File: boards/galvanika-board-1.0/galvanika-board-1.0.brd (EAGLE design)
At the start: 100 x 100 mm, 96 parts, among them IC1 LM358D, IC2 7805DT, IC3 74HCT595D, IC4 74HCT595D, IC5 74HCT595D, IC6 ATMEGA48/88/168-PU, IC7 74HC595D, Q1 20MHz

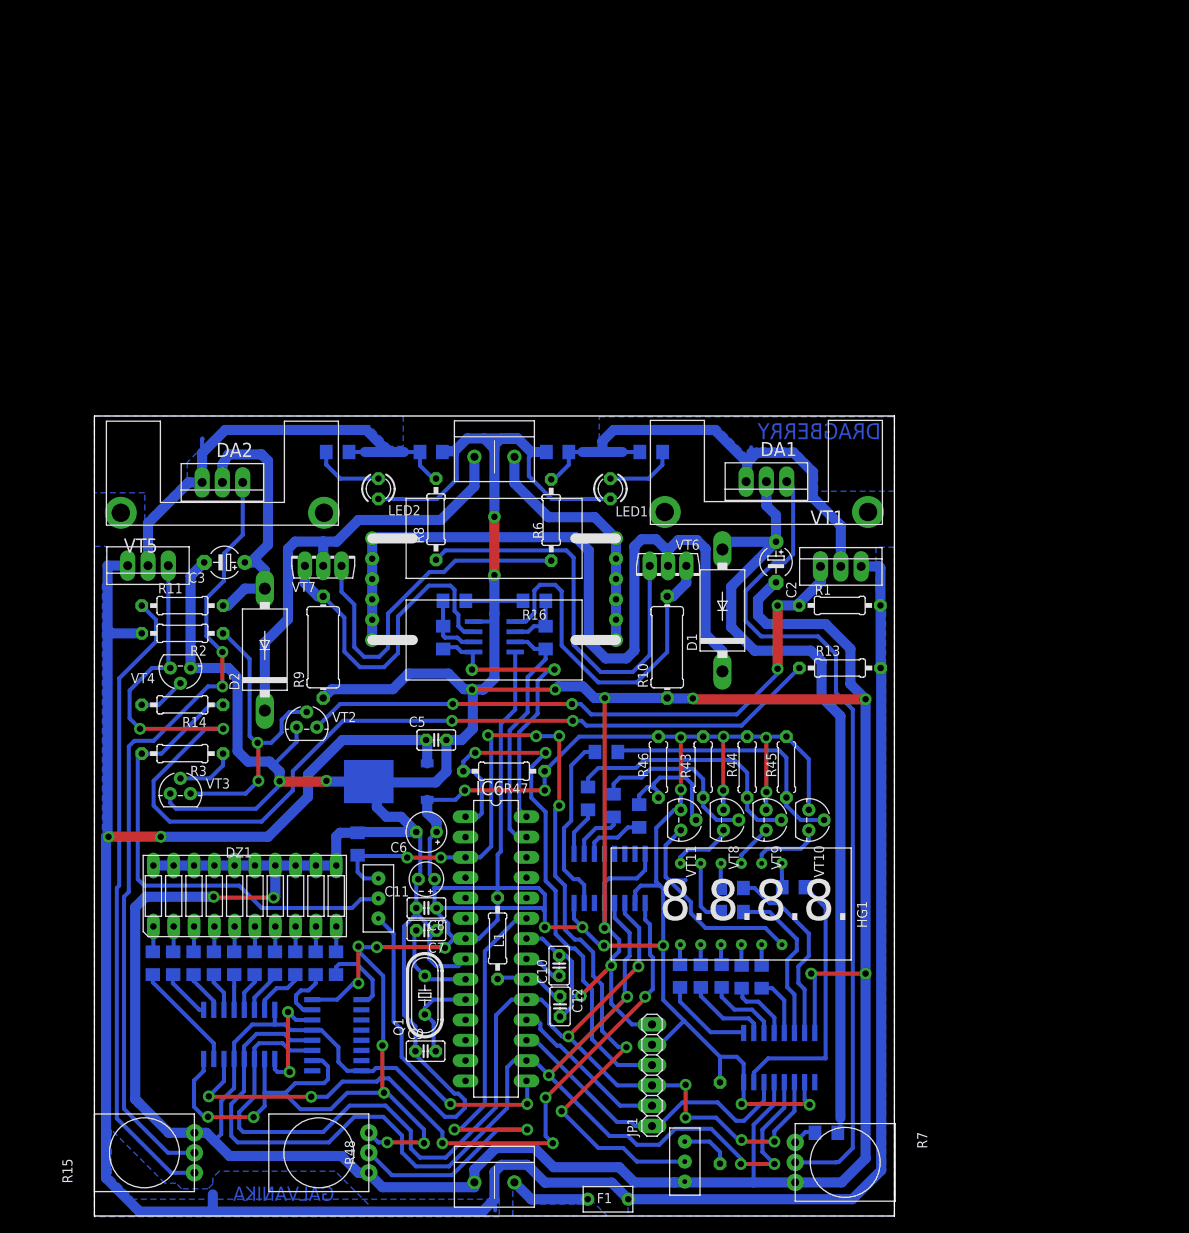
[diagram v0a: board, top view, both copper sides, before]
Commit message: new board version
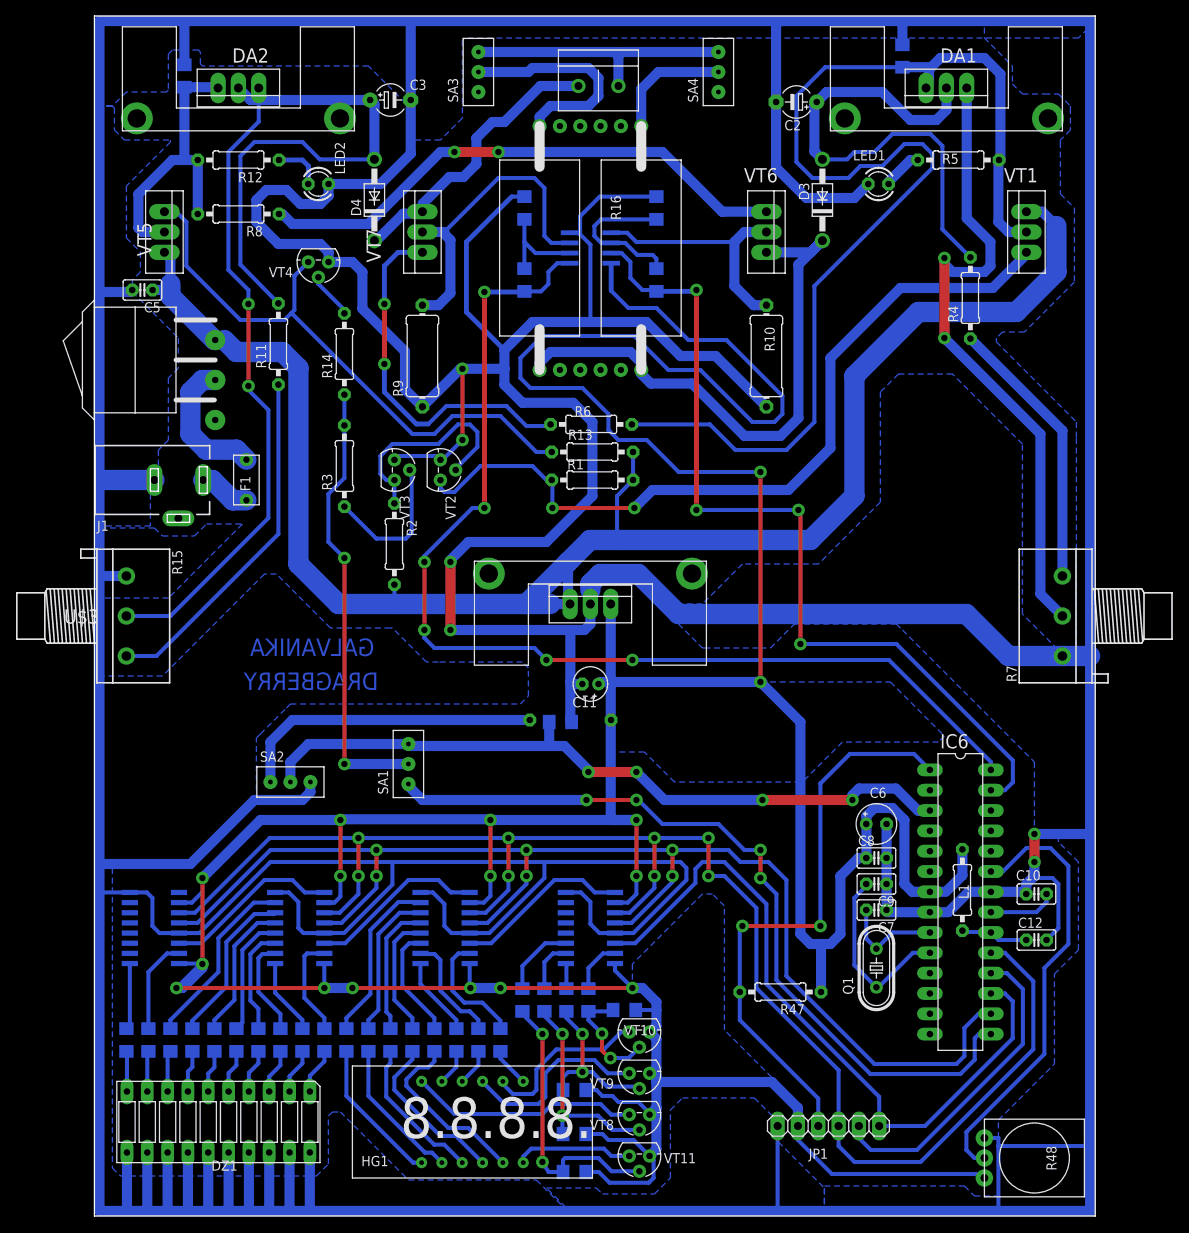
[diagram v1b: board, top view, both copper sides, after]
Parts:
- removed D1, D2: 1N5400, diode:DO201-15
- removed IC2: 7805DT, linear:TO252
- removed XS1: KLS2-2, dragberry:KLS2-2
- added D3, D4: 1N4001, tango:DO41-10
- added J1: (no value), con-jack:DCJ0303
- added SA3, SA4: (no value), dragberry:SS12D00
- added SA5: KCD11-101-H, dragberry:KCD11-101-H
- added U$3: L7805, dragberry:TO220-SK29-38S
- R12, R5: value 2K -> (none); device rcl:R1206 -> rcl:0207/10
- R15, R7: value 10K -> (none); device dragberry:R0904N -> pot:3RP/1610N
- R21, R22, R23, R24, R25, R26, R31, R32, R33, R34, R35, R36, R37, R38: value (none) -> 330
- R39, R40, R41, R42: value (none) -> 200
- R4: value 200 -> (none); device rcl:R1206 -> rcl:0207/10
- R43, R44, R45, R46: device rcl:0207/7 -> rcl:R1206
- VT6, VT7: value BD139 -> IRF1404; device dragberry:TO126AV -> dragberry:TO220-V
- moved R4 105.9 mm to (109.5, 114.8), flipped to the top, turned to 90 degrees
- moved F1 100.6 mm to (19.0, 92.0), turned to 90 degrees
- moved R48 77.0 mm to (111.2, 7.25), turned to 270 degrees
- moved R7 76.0 mm to (121.0, 75.0), turned to 90 degrees
- moved SA2 68.4 mm to (24.5, 54.2), turned to 0 degrees
- moved R15 67.6 mm to (4.00, 75.0), turned to 270 degrees
- moved C5 67.2 mm to (6.00, 115.8), turned to 180 degrees
- moved C1 65.6 mm to (101.0, 145.0), turned to 90 degrees
- moved C3 61.4 mm to (37.0, 139.5), turned to 0 degrees
- moved C10 60.3 mm to (117.8, 40.2), turned to 180 degrees
- moved C12 60.1 mm to (117.8, 34.5), turned to 0 degrees
- moved C9 60.1 mm to (97.8, 41.5), turned to 180 degrees
- moved L1 58.4 mm to (108.5, 40.8)
- moved IC6 58.3 mm to (108.2, 39.2)
- moved C2 57.6 mm to (87.8, 139.2), turned to 180 degrees
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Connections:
- net N$25 renamed BRANCH-CTRL
- net N$90 renamed RIGHT-EN
- removed net N$46: IC4.14
- removed net N$55: IC3.6, R31.1
- removed net N$91: F1.1, XS1.2
- new net N$60: D4.C, VT7.S, XS2.1
- new net N$62: F1.1, J1.1
- new net N$63: SA3.1$S, SA4.1$S, XS2.2
- new net N$65: F1.2, SA5.2
- new net N$66: IC4.14, IC6.17, JP1.1
- new net N$67: IC3.6, R34.1
- net +19V: now also SA5.3, U$3.1; no longer F1.2, IC2.1
- net A-LEFT: now also VT7.D; no longer VT7.E
- net A-RIGHT: now also VT6.D; no longer VT6.E
- net DATA: now also IC4.9; no longer IC6.17, JP1.1
- net GND: now also J1.3, R15.1, R7.1, U$3.2; no longer IC2.3, R15.3, R7.3, XS1.1
- net N$12: now also R8.1, VT6.G; no longer R6.2, VT7.B
- net N$13: now also D3.C, VT6.S; no longer D1.C, VT6.C
- net N$14: now also R16.2, SA3.1$P; no longer D2.C, VT7.C, XS2.1
- net N$15: now also R6.2, VT7.G; no longer R8.1, VT6.B
- net N$16: now also IC3.1, R31.1; no longer IC3.3, R38.1
- net N$17: now also IC3.7, R35.1; no longer IC3.2, R34.1
- net N$21: now also R15.3; no longer R15.1
- net N$3: now also SA4.1$P; no longer R16.2, XS2.2
- net N$35: now also R38.1; no longer R37.1
- net N$44: now also IC3.2; no longer IC3.7
- net N$45: now also IC3.9; no longer IC4.9
- net N$64: now also IC3.3, R37.1; no longer IC3.1, R35.1
- net N$9: now also R7.3; no longer R7.1
- net VCC: now also U$3.3; no longer IC2.2
- net VO-LEFT: now also D3.A; no longer D1.A
- net VO-RIGHT: now also D4.A; no longer D2.A
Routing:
- net GND: track 753.1 -> 1309.8 mm, vias 16 -> 6
- net VCC: track 378.3 -> 592.4 mm, vias 24 -> 16
- net +19V: track 321.0 -> 210.7 mm, vias 2 -> 0
- net N$28: track 37.9 -> 138.5 mm, vias 2 -> 6
- net N$66: track 0.00 -> 88.9 mm
- net VI-LEFT: track 61.9 -> 147.4 mm
- net N$11: track 31.0 -> 109.5 mm, vias 0 -> 4
- net N$45: track 90.0 -> 22.3 mm, vias 6 -> 0
- net N$20: track 140.8 -> 73.9 mm, vias 4 -> 0
- net PWM: track 39.8 -> 100.0 mm, vias 2 -> 4
- net CLOCK: track 146.6 -> 200.2 mm, vias 6 -> 8
- net VO-LEFT: track 102.4 -> 61.5 mm
- net N$60: track 0.00 -> 36.0 mm
- net N$21: track 79.4 -> 44.0 mm
- net N$63: track 0.00 -> 35.0 mm
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- added copper zone on layer 16, net GND
- added copper zone on layer 16, net VCC
- removed copper zone on layer 16, net +19V
- removed copper zone on layer 16, net N$91
- removed copper zone on layer 16, net VI-LEFT
- removed copper zone on layer 16, net VI-RIGHT
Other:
- board size 100 x 100 mm -> 125.1 x 150 mm
